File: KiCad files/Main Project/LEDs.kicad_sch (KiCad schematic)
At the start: 17 parts

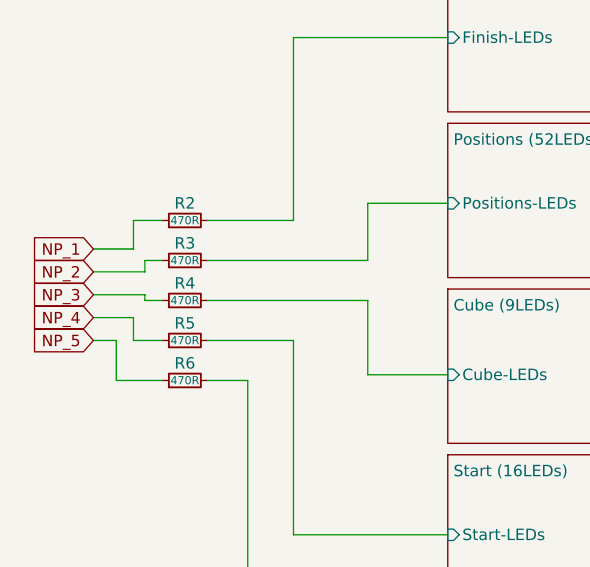
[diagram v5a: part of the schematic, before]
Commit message: update
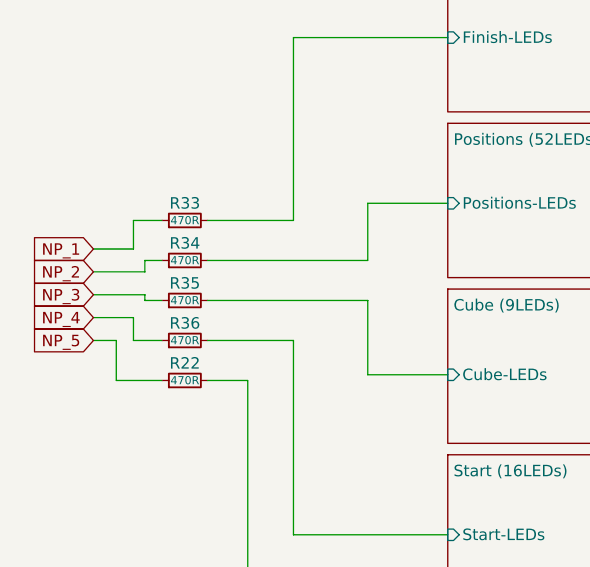
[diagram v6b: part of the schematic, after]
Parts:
- renumbered R6 to R22, R2 to R33, R3 to R34, R4 to R35, R5 to R36
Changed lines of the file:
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@@
   (symbol (lib_id "power:GND") (at 151.13 165.1 0) (unit 1)
     (in_bom yes) (on_board yes) (fields_autoplaced)
-    (property "Reference" "#PWR034" (id 0) (at 151.13 171.45 0)
+    (property "Reference" "#PWR0238" (id 0) (at 151.13 171.45 0)
       (effects (font (size 1.27 1.27)) hide)
     )
@@
   (symbol (lib_id "power:VCC") (at 232.41 118.745 0) (unit 1)
     (in_bom yes) (on_board yes) (fields_autoplaced)
-    (property "Reference" "#PWR018" (id 0) (at 232.41 122.555 0)
+    (property "Reference" "#PWR0255" (id 0) (at 232.41 122.555 0)
       (effects (font (size 1.27 1.27)) hide)
     )
@@
   (symbol (lib_id "power:GND") (at 130.81 133.985 0) (unit 1)
     (in_bom yes) (on_board yes) (fields_autoplaced)
-    (property "Reference" "#PWR021" (id 0) (at 130.81 140.335 0)
+    (property "Reference" "#PWR0252" (id 0) (at 130.81 140.335 0)
       (effects (font (size 1.27 1.27)) hide)
     )
@@
   (symbol (lib_id "power:GND") (at 151.13 133.985 0) (unit 1)
     (in_bom yes) (on_board yes) (fields_autoplaced)
-    (property "Reference" "#PWR022" (id 0) (at 151.13 140.335 0)
+    (property "Reference" "#PWR0248" (id 0) (at 151.13 140.335 0)
       (effects (font (size 1.27 1.27)) hide)
     )
@@
   (symbol (lib_id "power:GND") (at 90.17 133.985 0) (unit 1)
     (in_bom yes) (on_board yes) (fields_autoplaced)
-    (property "Reference" "#PWR019" (id 0) (at 90.17 140.335 0)
+    (property "Reference" "#PWR0234" (id 0) (at 90.17 140.335 0)
       (effects (font (size 1.27 1.27)) hide)
     )
@@
   (symbol (lib_id "Device:R_Small") (at 52.07 60.325 90) (unit 1)
     (in_bom yes) (on_board yes)
-    (property "Reference" "R3" (id 0) (at 52.07 58.42 90))
+    (property "Reference" "R34" (id 0) (at 52.07 58.42 90))
     (property "Value" "470R" (id 1) (at 52.07 60.325 90)
       (effects (font (size 0.9 0.9)))
@@
   (symbol (lib_id "power:GND") (at 110.49 165.1 0) (unit 1)
     (in_bom yes) (on_board yes) (fields_autoplaced)
-    (property "Reference" "#PWR032" (id 0) (at 110.49 171.45 0)
+    (property "Reference" "#PWR0240" (id 0) (at 110.49 171.45 0)
       (effects (font (size 1.27 1.27)) hide)
     )
@@
   (symbol (lib_id "power:VCC") (at 212.09 118.745 0) (unit 1)
     (in_bom yes) (on_board yes) (fields_autoplaced)
-    (property "Reference" "#PWR017" (id 0) (at 212.09 122.555 0)
+    (property "Reference" "#PWR0247" (id 0) (at 212.09 122.555 0)
       (effects (font (size 1.27 1.27)) hide)
     )
@@
   (symbol (lib_id "power:GND") (at 110.49 133.985 0) (unit 1)
     (in_bom yes) (on_board yes) (fields_autoplaced)
-    (property "Reference" "#PWR020" (id 0) (at 110.49 140.335 0)
+    (property "Reference" "#PWR0235" (id 0) (at 110.49 140.335 0)
       (effects (font (size 1.27 1.27)) hide)
     )
@@
   (symbol (lib_id "power:VCC") (at 151.13 149.86 0) (unit 1)
     (in_bom yes) (on_board yes) (fields_autoplaced)
-    (property "Reference" "#PWR030" (id 0) (at 151.13 153.67 0)
+    (property "Reference" "#PWR0236" (id 0) (at 151.13 153.67 0)
       (effects (font (size 1.27 1.27)) hide)
     )
@@
   (symbol (lib_id "power:VCC") (at 151.13 118.745 0) (unit 1)
     (in_bom yes) (on_board yes) (fields_autoplaced)
-    (property "Reference" "#PWR014" (id 0) (at 151.13 122.555 0)
+    (property "Reference" "#PWR0243" (id 0) (at 151.13 122.555 0)
       (effects (font (size 1.27 1.27)) hide)
     )
@@
   (symbol (lib_id "power:VCC") (at 171.45 118.745 0) (unit 1)
     (in_bom yes) (on_board yes) (fields_autoplaced)
-    (property "Reference" "#PWR015" (id 0) (at 171.45 122.555 0)
+    (property "Reference" "#PWR0249" (id 0) (at 171.45 122.555 0)
       (effects (font (size 1.27 1.27)) hide)
     )
@@
   (symbol (lib_id "power:VCC") (at 90.17 149.86 0) (unit 1)
     (in_bom yes) (on_board yes) (fields_autoplaced)
-    (property "Reference" "#PWR027" (id 0) (at 90.17 153.67 0)
+    (property "Reference" "#PWR0233" (id 0) (at 90.17 153.67 0)
       (effects (font (size 1.27 1.27)) hide)
     )
@@
   (symbol (lib_id "power:GND") (at 130.81 165.1 0) (unit 1)
     (in_bom yes) (on_board yes) (fields_autoplaced)
-    (property "Reference" "#PWR033" (id 0) (at 130.81 171.45 0)
+    (property "Reference" "#PWR0239" (id 0) (at 130.81 171.45 0)
       (effects (font (size 1.27 1.27)) hide)
     )
@@
   (symbol (lib_id "power:GND") (at 232.41 133.985 0) (unit 1)
     (in_bom yes) (on_board yes) (fields_autoplaced)
-    (property "Reference" "#PWR026" (id 0) (at 232.41 140.335 0)
+    (property "Reference" "#PWR0254" (id 0) (at 232.41 140.335 0)
       (effects (font (size 1.27 1.27)) hide)
     )
@@
   (symbol (lib_id "power:GND") (at 90.17 165.1 0) (unit 1)
     (in_bom yes) (on_board yes) (fields_autoplaced)
-    (property "Reference" "#PWR031" (id 0) (at 90.17 171.45 0)
+    (property "Reference" "#PWR0232" (id 0) (at 90.17 171.45 0)
       (effects (font (size 1.27 1.27)) hide)
     )
@@
   (symbol (lib_id "power:VCC") (at 130.81 118.745 0) (unit 1)
     (in_bom yes) (on_board yes) (fields_autoplaced)
-    (property "Reference" "#PWR013" (id 0) (at 130.81 122.555 0)
+    (property "Reference" "#PWR0242" (id 0) (at 130.81 122.555 0)
       (effects (font (size 1.27 1.27)) hide)
     )
@@
   (symbol (lib_id "power:VCC") (at 90.17 118.745 0) (unit 1)
     (in_bom yes) (on_board yes) (fields_autoplaced)
-    (property "Reference" "#PWR011" (id 0) (at 90.17 122.555 0)
+    (property "Reference" "#PWR0245" (id 0) (at 90.17 122.555 0)
       (effects (font (size 1.27 1.27)) hide)
     )
@@
   (symbol (lib_id "power:VCC") (at 110.49 149.86 0) (unit 1)
     (in_bom yes) (on_board yes) (fields_autoplaced)
-    (property "Reference" "#PWR028" (id 0) (at 110.49 153.67 0)
+    (property "Reference" "#PWR0241" (id 0) (at 110.49 153.67 0)
       (effects (font (size 1.27 1.27)) hide)
     )
@@
   (symbol (lib_id "power:VCC") (at 110.49 118.745 0) (unit 1)
     (in_bom yes) (on_board yes) (fields_autoplaced)
-    (property "Reference" "#PWR012" (id 0) (at 110.49 122.555 0)
+    (property "Reference" "#PWR0244" (id 0) (at 110.49 122.555 0)
       (effects (font (size 1.27 1.27)) hide)
     )
@@
   (symbol (lib_id "Device:R_Small") (at 52.07 73.66 90) (unit 1)
     (in_bom yes) (on_board yes)
-    (property "Reference" "R6" (id 0) (at 52.07 71.755 90))
+    (property "Reference" "R22" (id 0) (at 52.07 71.755 90))
     (property "Value" "470R" (id 1) (at 52.07 73.66 90)
       (effects (font (size 0.9 0.9)))
@@
   (symbol (lib_id "power:GND") (at 191.77 133.985 0) (unit 1)
     (in_bom yes) (on_board yes) (fields_autoplaced)
-    (property "Reference" "#PWR024" (id 0) (at 191.77 140.335 0)
+    (property "Reference" "#PWR0251" (id 0) (at 191.77 140.335 0)
       (effects (font (size 1.27 1.27)) hide)
     )
@@
   (symbol (lib_id "power:GND") (at 171.45 133.985 0) (unit 1)
     (in_bom yes) (on_board yes) (fields_autoplaced)
-    (property "Reference" "#PWR023" (id 0) (at 171.45 140.335 0)
+    (property "Reference" "#PWR0250" (id 0) (at 171.45 140.335 0)
       (effects (font (size 1.27 1.27)) hide)
     )
@@
   (symbol (lib_id "power:VCC") (at 191.77 118.745 0) (unit 1)
     (in_bom yes) (on_board yes) (fields_autoplaced)
-    (property "Reference" "#PWR016" (id 0) (at 191.77 122.555 0)
+    (property "Reference" "#PWR0253" (id 0) (at 191.77 122.555 0)
       (effects (font (size 1.27 1.27)) hide)
     )
@@
   (symbol (lib_id "power:GND") (at 212.09 133.985 0) (unit 1)
     (in_bom yes) (on_board yes) (fields_autoplaced)
-    (property "Reference" "#PWR025" (id 0) (at 212.09 140.335 0)
+    (property "Reference" "#PWR0246" (id 0) (at 212.09 140.335 0)
       (effects (font (size 1.27 1.27)) hide)
     )
@@
   (symbol (lib_id "Device:R_Small") (at 52.07 69.215 90) (unit 1)
     (in_bom yes) (on_board yes)
-    (property "Reference" "R5" (id 0) (at 52.07 67.31 90))
+    (property "Reference" "R36" (id 0) (at 52.07 67.31 90))
     (property "Value" "470R" (id 1) (at 52.07 69.215 90)
       (effects (font (size 0.9 0.9)))
@@
   (symbol (lib_id "Device:R_Small") (at 52.07 55.88 90) (unit 1)
     (in_bom yes) (on_board yes)
-    (property "Reference" "R2" (id 0) (at 52.07 53.975 90))
+    (property "Reference" "R33" (id 0) (at 52.07 53.975 90))
     (property "Value" "470R" (id 1) (at 52.07 55.88 90)
       (effects (font (size 0.9 0.9)))
@@
   (symbol (lib_id "power:VCC") (at 130.81 149.86 0) (unit 1)
     (in_bom yes) (on_board yes) (fields_autoplaced)
-    (property "Reference" "#PWR029" (id 0) (at 130.81 153.67 0)
+    (property "Reference" "#PWR0237" (id 0) (at 130.81 153.67 0)
       (effects (font (size 1.27 1.27)) hide)
     )
@@
   (symbol (lib_id "Device:R_Small") (at 52.07 64.77 90) (unit 1)
     (in_bom yes) (on_board yes)
-    (property "Reference" "R4" (id 0) (at 52.07 62.865 90))
+    (property "Reference" "R35" (id 0) (at 52.07 62.865 90))
     (property "Value" "470R" (id 1) (at 52.07 64.77 90)
       (effects (font (size 0.9 0.9)))
